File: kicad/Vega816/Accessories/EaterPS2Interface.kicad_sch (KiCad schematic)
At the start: 14 parts, among them J102 VIA Port

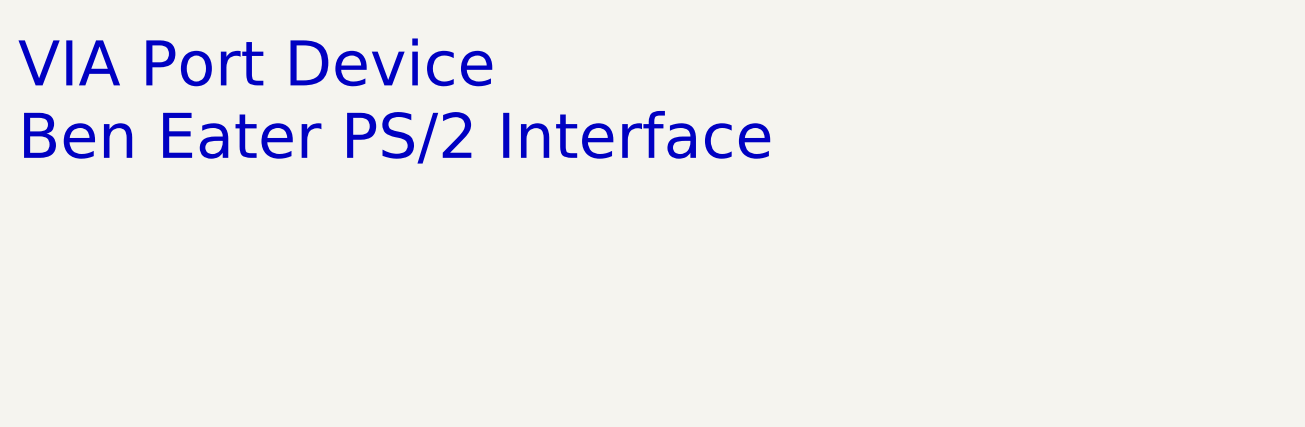
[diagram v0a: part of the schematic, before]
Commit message: update
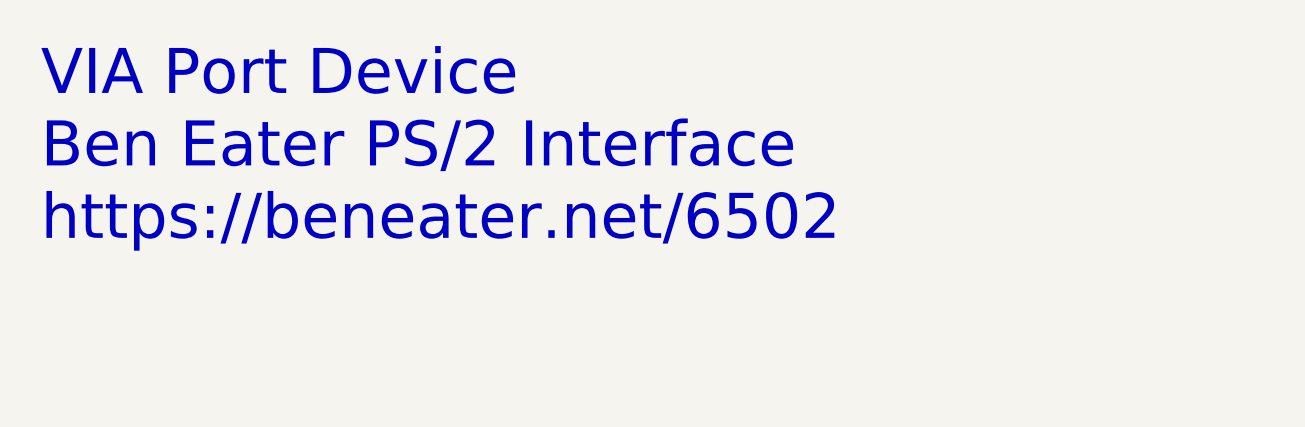
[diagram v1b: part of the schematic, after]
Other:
- note added: "VIA Port Device Ben Eater PS/2 Interface https://beneater.net/6502"
- note removed: "VIA Port Device Ben Eater PS/2 Interface"
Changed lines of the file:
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@@
     (stroke (width 0) (type default) (color 0 0 0 0))
   )
-  (text "VIA Port Device\nBen Eater PS/2 Interface\n" (at 16.51 34.29 0)
+  (text "VIA Port Device\nBen Eater PS/2 Interface\nhttps://beneater.net/6502\n"
+    (at 19.05 43.18 0)
     (effects (font (size 5 5)) (justify left bottom))
   )
